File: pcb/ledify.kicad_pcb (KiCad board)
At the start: 0 parts

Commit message: finished stuff
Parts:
- added AE1: Antenna_Shield, RF_Antenna:Texas_SWRA117D_2.4GHz_Right, F.Cu at (75.9, 41.9)
- added C1: 4.7uF 50V, Capacitor_SMD:C_0603_1608Metric, F.Cu at (80.4, 76.8)
- added C10: 22uF, Capacitor_SMD:C_1210_3225Metric, F.Cu at (62.0, 51.8)
- added C11: 22uF, Capacitor_SMD:C_1210_3225Metric, F.Cu at (60.9, 48.2)
- added C12: 22uF, Capacitor_SMD:C_1210_3225Metric, F.Cu at (56.9, 51.8)
- added C13: 22uF, Capacitor_SMD:C_1210_3225Metric, F.Cu at (62.0, 55.2)
- added C14: 22uF, Capacitor_SMD:C_1210_3225Metric, F.Cu at (56.9, 55.2)
- added C15: 10uF, Capacitor_SMD:C_0805_2012Metric, F.Cu at (76.8, 76.6)
- added C16: 100nF, Capacitor_SMD:C_0402_1005Metric, F.Cu at (76.6, 70.9)
- added C17: 22uF, Capacitor_SMD:C_0805_2012Metric, F.Cu at (75.5, 64.2)
- added C18: 22uF, Capacitor_SMD:C_0805_2012Metric, F.Cu at (78.9, 64.2)
- added C19: 100nF, Capacitor_SMD:C_0402_1005Metric, F.Cu at (76.6, 85.5)
- added C2: 400pF, Capacitor_SMD:C_0402_1005Metric, F.Cu at (75.6, 82.3)
- added C20: 100nF, Capacitor_SMD:C_0402_1005Metric, F.Cu at (76.6, 83.6)
- added C21: 1uF, Capacitor_SMD:C_0402_1005Metric, F.Cu at (72.6, 82.0)
- added C22: 12pF, Capacitor_SMD:C_0402_1005Metric, F.Cu at (82.6, 46.4)
- added C23: 12pF, Capacitor_SMD:C_0402_1005Metric, F.Cu at (87.7, 46.9)
- added C24: 100nF, Capacitor_SMD:C_0402_1005Metric, F.Cu at (87.5, 54.6)
- added C25: 1uF, Capacitor_SMD:C_0402_1005Metric, F.Cu at (87.5, 53.6)
- added C26: 100nF, Capacitor_SMD:C_0402_1005Metric, F.Cu at (77.4, 53.4)
- added C27: 100nF, Capacitor_SMD:C_0402_1005Metric, F.Cu at (86.4, 49.8)
- added C28: 1uF, Capacitor_SMD:C_0402_1005Metric, F.Cu at (75.0, 52.9)
- added C29: 10uF, Capacitor_SMD:C_0603_1608Metric, F.Cu at (73.8, 51.5)
- added C3: 400pF, Capacitor_SMD:C_0402_1005Metric, F.Cu at (75.6, 86.6)
- added C30: 100nF, Capacitor_SMD:C_0402_1005Metric, F.Cu at (76.0, 52.9)
- added C31: 100nF, Capacitor_SMD:C_0402_1005Metric, F.Cu at (79.0, 50.8)
- added C32: 10nF, Capacitor_SMD:C_0402_1005Metric, F.Cu at (81.0, 47.7)
- added C33: 1uF, Capacitor_SMD:C_0402_1005Metric, F.Cu at (83.0, 48.6)
- added C34: 17pF, Capacitor_SMD:C_0402_1005Metric, F.Cu at (75.9, 54.8)
- added C35: 17pF, Capacitor_SMD:C_0402_1005Metric, F.Cu at (75.9, 56.7)
- added C36: 1uF, Capacitor_SMD:C_0603_1608Metric, F.Cu at (77.8, 52.4)
- added C37: 100nF, Capacitor_SMD:C_0402_1005Metric, F.Cu at (76.4, 60.1)
- added C38: 100nF, Capacitor_SMD:C_0402_1005Metric, F.Cu at (76.7, 58.7)
- added C39: 100nF, Capacitor_SMD:C_0402_1005Metric, F.Cu at (81.3, 56.4)
- added C4: 100nF, Capacitor_SMD:C_0402_1005Metric_Pad0.74x0.62mm_HandSolder, F.Cu at (60.4, 80.7)
- added C40: 100nF, Capacitor_SMD:C_0402_1005Metric, F.Cu at (81.9, 57.8)
- added C41: 4pF, Capacitor_SMD:C_0402_1005Metric, F.Cu at (79.0, 46.4)
- added C42: 4.6pF, Capacitor_SMD:C_0402_1005Metric, F.Cu at (79.0, 48.9)
- added C5: 10uF 50V, Capacitor_SMD:C_0805_2012Metric, F.Cu at (68.4, 78.8)
- added C6: 470nF, Capacitor_SMD:C_0603_1608Metric, F.Cu at (66.6, 79.0)
- added C7: 10uF 50V, Capacitor_SMD:C_0805_2012Metric, F.Cu at (59.0, 78.5)
- added C8: 470nF, Capacitor_SMD:C_0603_1608Metric, F.Cu at (60.8, 78.7)
- added C9: 1uF, Capacitor_SMD:C_0603_1608Metric, F.Cu at (63.1, 83.8)
- added H1: MountingHole, MountingHole:MountingHole_2.2mm_M2_Pad_Via, F.Cu at (57.4, 85.2)
- added J1: Conn_01x01_Pin, Connector_Wire:SolderWirePad_1x01_SMD_3x6mm, F.Cu at (57.5, 39.6)
- added J2: USB_C_Receptacle_USB2.0_16P, Connector_USB:USB_C_Receptacle_HCTL_HC-TYPE-C-16P-01A, F.Cu at (83.4, 85.9)
- added J3: Conn_01x01_Pin, Connector_Wire:SolderWirePad_1x01_SMD_3x6mm, F.Cu at (62.7, 39.6)
- added J4: Conn_01x01_Pin, Connector_Wire:SolderWirePad_1x01_SMD_3x6mm, F.Cu at (68.0, 39.6)
- added L1: ZEMS1770-6R8M, lcsc:IND-SMD_L17.5-W17.5_SLO1770H, F.Cu at (63.7, 67.0)
- added L2: XRCD43-3R9M, lcsc:IND-SMD_L4.0-W3.2_XRCD43, F.Cu at (77.1, 67.7)
- added L3: VHF160808H2N0ST, lcsc:L0603, F.Cu at (77.3, 51.3)
- added L5: TCGL1005B1N8SAT, lcsc:L0402, F.Cu at (79.5, 47.7)
- added Q1: 2N7002K, Package_TO_SOT_SMD:SOT-23, F.Cu at (65.6, 85.8)
- added R1: 100K, Resistor_SMD:R_0402_1005Metric, F.Cu at (67.0, 83.5)
- added R2: 100K, Resistor_SMD:R_0402_1005Metric, F.Cu at (62.6, 85.1)
- added R3: 24.9K, Resistor_SMD:R_0402_1005Metric, F.Cu at (62.1, 86.5)
- added R4: 14.3K, Resistor_SMD:R_0402_1005Metric, F.Cu at (63.1, 86.5)
- added R5: 4.7K, Resistor_SMD:R_0402_1005Metric, F.Cu at (71.2, 83.6)
- added R6: 4.7K, Resistor_SMD:R_0402_1005Metric, F.Cu at (69.6, 84.1)
- added R7: 4.7K, Resistor_SMD:R_0402_1005Metric, F.Cu at (71.2, 85.8)
- added R8: 4.7K, Resistor_SMD:R_0402_1005Metric, F.Cu at (88.4, 64.5)
- added R9: 4.7K, Resistor_SMD:R_0402_1005Metric, F.Cu at (68.1, 86.2)
- added SW1: TS-1088-AR02016, lcsc:SW-SMD_L3.9-W3.0-P4.45, F.Cu at (86.8, 67.6)
- added SW2: TS-1088-AR02016, lcsc:SW-SMD_L3.9-W3.0-P4.45, F.Cu at (86.8, 74.8)
- added U1: ESP32-C6_C5364646, lcsc:QFN-40_L5.0-W5.0-P0.40-TL-EP3.3, F.Cu at (83.0, 52.4)
- added U2: USBLC6-2P6, Package_TO_SOT_SMD:SOT-666, F.Cu at (83.5, 79.2)
- added U3: AP63203WU, Package_TO_SOT_SMD:TSOT-23-6, F.Cu at (77.1, 73.5)
- added U4: FUSB302BMPX, Package_DFN_QFN:WQFN-14-1EP_2.5x2.5mm_P0.5mm_EP1.45x1.45mm, F.Cu at (73.5, 84.5)
- added U5: W25Q128JVP, Package_SON:WSON-8-1EP_6x5mm_P1.27mm_EP3.4x4.3mm, F.Cu at (86.7, 59.5)
- added U6: LM61495QRPHRQ1, lcsc:VQFN-16_L4.5-W3.5-P0.50-TL_TI_RPH, F.Cu at (63.7, 80.7)
- added U7: BMI323, lcsc:LGA-14_L3.0-W2.5-P0.50-TL_QMI8658A, F.Cu at (74.4, 60.1)
- added U8: BMP581, lcsc:LGA-10_L2.0-W2.0-P0.50-TL_BMP581, F.Cu at (80.4, 57.9)
- added X1: XL2EL89COI-111YLC-40M, lcsc:CRYSTAL-SMD_4P-L3.2-W2.5-BL, F.Cu at (85.6, 46.9)
- added X2: Q13FC1350000400, lcsc:FC-135R_L3.2-W1.5, F.Cu at (77.4, 55.8)
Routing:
- net +3V3: track 0.00 -> 57.5 mm, vias 0 -> 28
- net LED_VCC: track 0.00 -> 46.4 mm, vias 0 -> 3
- net /LED_SW_V: track 0.00 -> 45.1 mm, vias 0 -> 4
- net /LED_ENABLE: track 0.00 -> 41.6 mm, vias 0 -> 4
- net /LED_CON: track 0.00 -> 33.8 mm, vias 0 -> 2
- net /CHIP_EN: track 0.00 -> 29.0 mm, vias 0 -> 2
- net /CHIP_BOOT: track 0.00 -> 24.0 mm, vias 0 -> 3
- net /DP: track 0.00 -> 24.0 mm
- net /DN: track 0.00 -> 24.0 mm
- net VBUS: track 0.00 -> 22.3 mm, vias 0 -> 48
- net GND: track 0.00 -> 21.4 mm, vias 0 -> 273
- net /SPI_MISO: track 0.00 -> 20.4 mm, vias 0 -> 3
- net /SPI_MOSI: track 0.00 -> 20.1 mm, vias 0 -> 3
- net /SPI_SCK: track 0.00 -> 18.2 mm, vias 0 -> 3
- net /CS_IMU: track 0.00 -> 17.6 mm, vias 0 -> 2
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- added copper zone on F.Cu, net +3V3
- added copper zone on In2.Cu, net +3V3
- added copper zone on B.Cu, net GND
- added copper zone on F.Cu, net GND
- added copper zone on In1.Cu, net GND
- added copper zone on F.Cu, net LED_VCC
- added copper zone on In1.Cu, net LED_VCC
- added copper zone on F.Cu, net Net-(U6-SW)
- added copper zone on F.Cu, net VBUS
- added copper zone on In2.Cu, net VBUS
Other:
- board outline added: 35.5 x 52.5 mm
- copper layers 0 -> 4
- board text added: "BOOT"
- board text added: "GND"
- board text added: "LEDIFY"
- board text added: "RST"
- board text added: "SIG"
- board text added: "VCC"

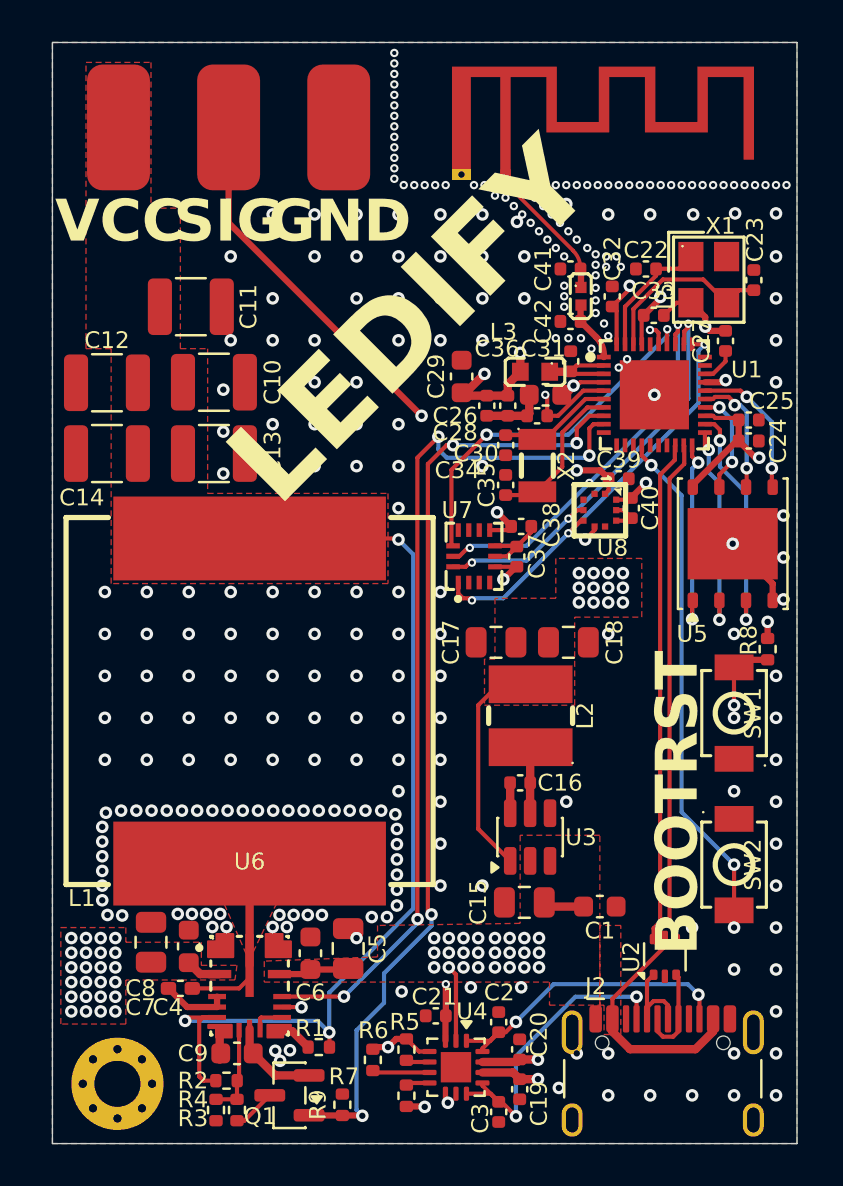
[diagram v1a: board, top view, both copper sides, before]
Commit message: finish prod
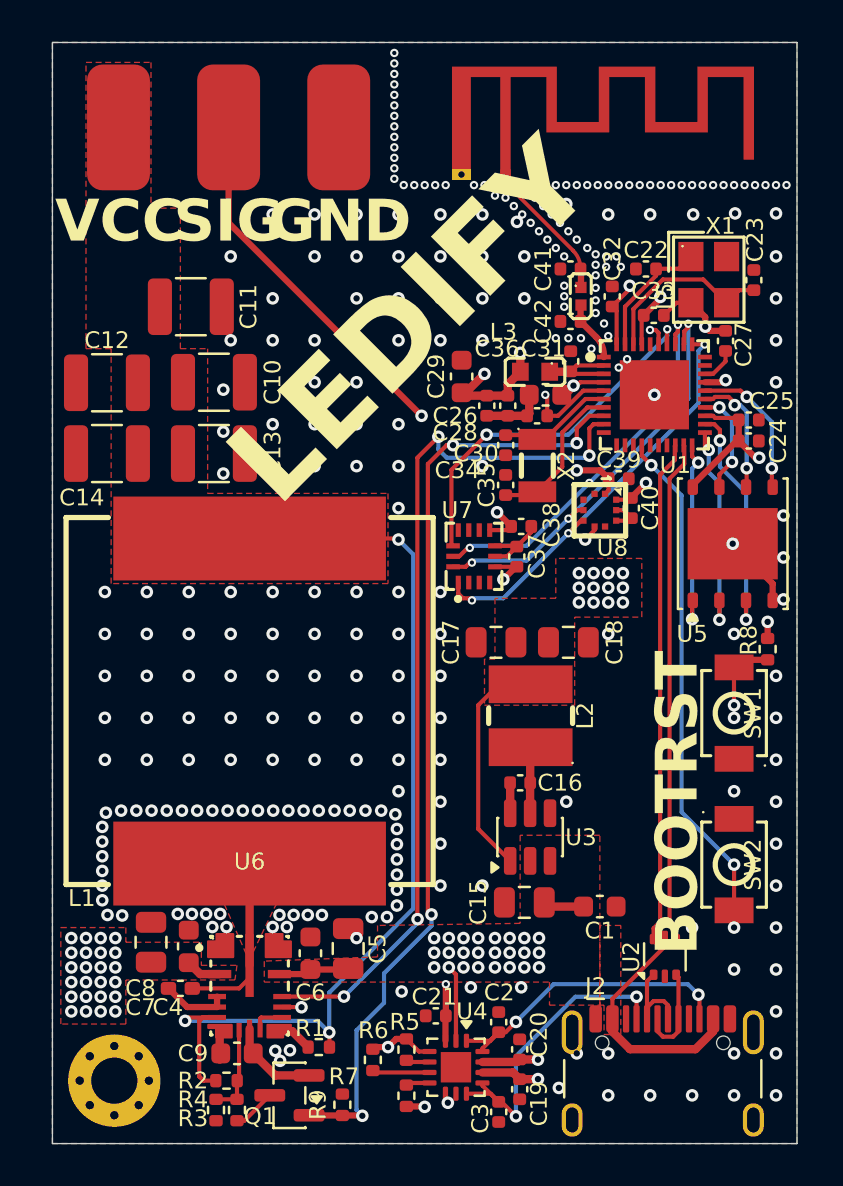
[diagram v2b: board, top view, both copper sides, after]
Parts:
- moved H1 0.21 mm to (57.2, 85.1)

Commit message: aaa
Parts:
- C10, C11, C12, C13, C14: value 22uF -> 22uF 25V
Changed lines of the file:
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@@
 			)
 		)
-		(property "Value" "22uF"
+		(property "Value" "22uF\n25V"
 			(at 0 2.3 0)
 			(layer "F.Fab")
@@
 			)
 		)
+		(property "LCSC" "C309062"
+			(at 0 0 0)
+			(unlocked yes)
+			(layer "F.Fab")
+			(hide yes)
+			(effects
+				(font
+					(size 1 1)
+					(thickness 0.15)
+				)
+			)
+		)
 		(property ki_fp_filters "C_*")
 		(sheetname "/")
@@
 			)
 		)
+		(property "LCSC" "C541337"
+			(at 0 0 180)
+			(unlocked yes)
+			(layer "F.Fab")
+			(hide yes)
+			(effects
+				(font
+					(size 1 1)
+					(thickness 0.15)
+				)
+			)
+		)
 		(property ki_fp_filters "C_*")
 		(sheetname "/")
@@
 			)
 		)
+		(property "LCSC" "C2441427"
+			(at 0 0 90)
+			(unlocked yes)
+			(layer "F.Fab")
+			(hide yes)
+			(effects
+				(font
+					(size 1 1)
+					(thickness 0.15)
+				)
+			)
+		)
 		(property ki_fp_filters "WSON*1EP*6x5mm*P1.27mm*EP3.4x4.3mm*")
 		(sheetname "/")
@@
 			)
 		)
+		(property "LCSC" "C780769"
+			(at 0 0 90)
+			(unlocked yes)
+			(layer "F.Fab")
+			(hide yes)
+			(effects
+				(font
+					(size 1 1)
+					(thickness 0.15)
+				)
+			)
+		)
 		(property ki_fp_filters "TSOT?23*")
 		(sheetname "/")
@@
 			)
 		)
-		(property "Value" "22uF"
+		(property "Value" "22uF\n25V"
 			(at 0 2.3 0)
 			(layer "F.Fab")
@@
 			)
 		)
+		(property "LCSC" "C309062"
+			(at 0 0 0)
+			(unlocked yes)
+			(layer "F.Fab")
+			(hide yes)
+			(effects
+				(font
+					(size 1 1)
+					(thickness 0.15)
+				)
+			)
+		)
 		(property ki_fp_filters "C_*")
 		(sheetname "/")
@@
 			)
 		)
-		(property "Value" "22uF"
+		(property "Value" "22uF\n25V"
 			(at 0 2.3 180)
 			(layer "F.Fab")
@@
 			)
 		)
+		(property "LCSC" "C309062"
+			(at 0 0 180)
+			(unlocked yes)
+			(layer "F.Fab")
+			(hide yes)
+			(effects
+				(font
+					(size 1 1)
+					(thickness 0.15)
+				)
+			)
+		)
 		(property ki_fp_filters "C_*")
 		(sheetname "/")
@@
 			)
 		)
+		(property "LCSC" "C76971"
+			(at 0 0 90)
+			(unlocked yes)
+			(layer "F.Fab")
+			(hide yes)
+			(effects
+				(font
+					(size 1 1)
+					(thickness 0.15)
+				)
+			)
+		)
 		(property ki_fp_filters "C_*")
 		(sheetname "/")
@@
 			)
 		)
+		(property "LCSC" "C1855288"
+			(at 0 0 180)
+			(unlocked yes)
+			(layer "F.Fab")
+			(hide yes)
+			(effects
+				(font
+					(size 1 1)
+					(thickness 0.15)
+				)
+			)
+		)
 		(property ki_fp_filters "C_*")
 		(sheetname "/")
@@
 			)
 		)
-		(property "Value" "22uF"
+		(property "Value" "22uF\n25V"
 			(at 0 2.3 180)
 			(layer "F.Fab")
@@
 			)
 		)
+		(property "LCSC" "C309062"
+			(at 0 0 180)
+			(unlocked yes)
+			(layer "F.Fab")
+			(hide yes)
+			(effects
+				(font
+					(size 1 1)
+					(thickness 0.15)
+				)
+			)
+		)
 		(property ki_fp_filters "C_*")
 		(sheetname "/")
@@
 			)
 		)
+		(property "LCSC" "C76971"
+			(at 0 0 270)
+			(unlocked yes)
+			(layer "F.Fab")
+			(hide yes)
+			(effects
+				(font
+					(size 1 1)
+					(thickness 0.15)
+				)
+			)
+		)
 		(property ki_fp_filters "C_*")
 		(sheetname "/")
@@
 			)
 		)
+		(property "LCSC" "C2894897"
+			(at 0 0 0)
+			(unlocked yes)
+			(layer "F.Fab")
+			(hide yes)
+			(effects
+				(font
+					(size 1 1)
+					(thickness 0.15)
+				)
+			)
+		)
 		(property ki_fp_filters "USB*C*Receptacle*")
 		(sheetname "/")
@@
 			)
 		)
-		(property "Value" "22uF"
+		(property "Value" "22uF\n25V"
 			(at 0 2.3 0)
 			(layer "F.Fab")
@@
 			(hide yes)
 			(effects
+				(font
+					(size 1 1)
+					(thickness 0.15)
+				)
+			)
+		)
+		(property "LCSC" "C309062"
+			(at 0 0 0)
+			(unlocked yes)
+			(layer "F.Fab")
+			(hide yes)
+			(effects
